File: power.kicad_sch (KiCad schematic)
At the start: 27 parts, among them J14 DeployLipo, J15 UCLipo, Q10 AO3401A, Q7 SI4143DY-T1-GE3, Q8 SI4143DY-T1-GE3, Q9 AO3401A, U10 LTC4411ES5TRMPBF, U11 LTC4411ES5TRMPBF, U12 LT1963AxST-3.3, U13 LTC4412xS6, U14 LTC4412xS6, U15 LTC4412xS6, U16 LTC4412xS6

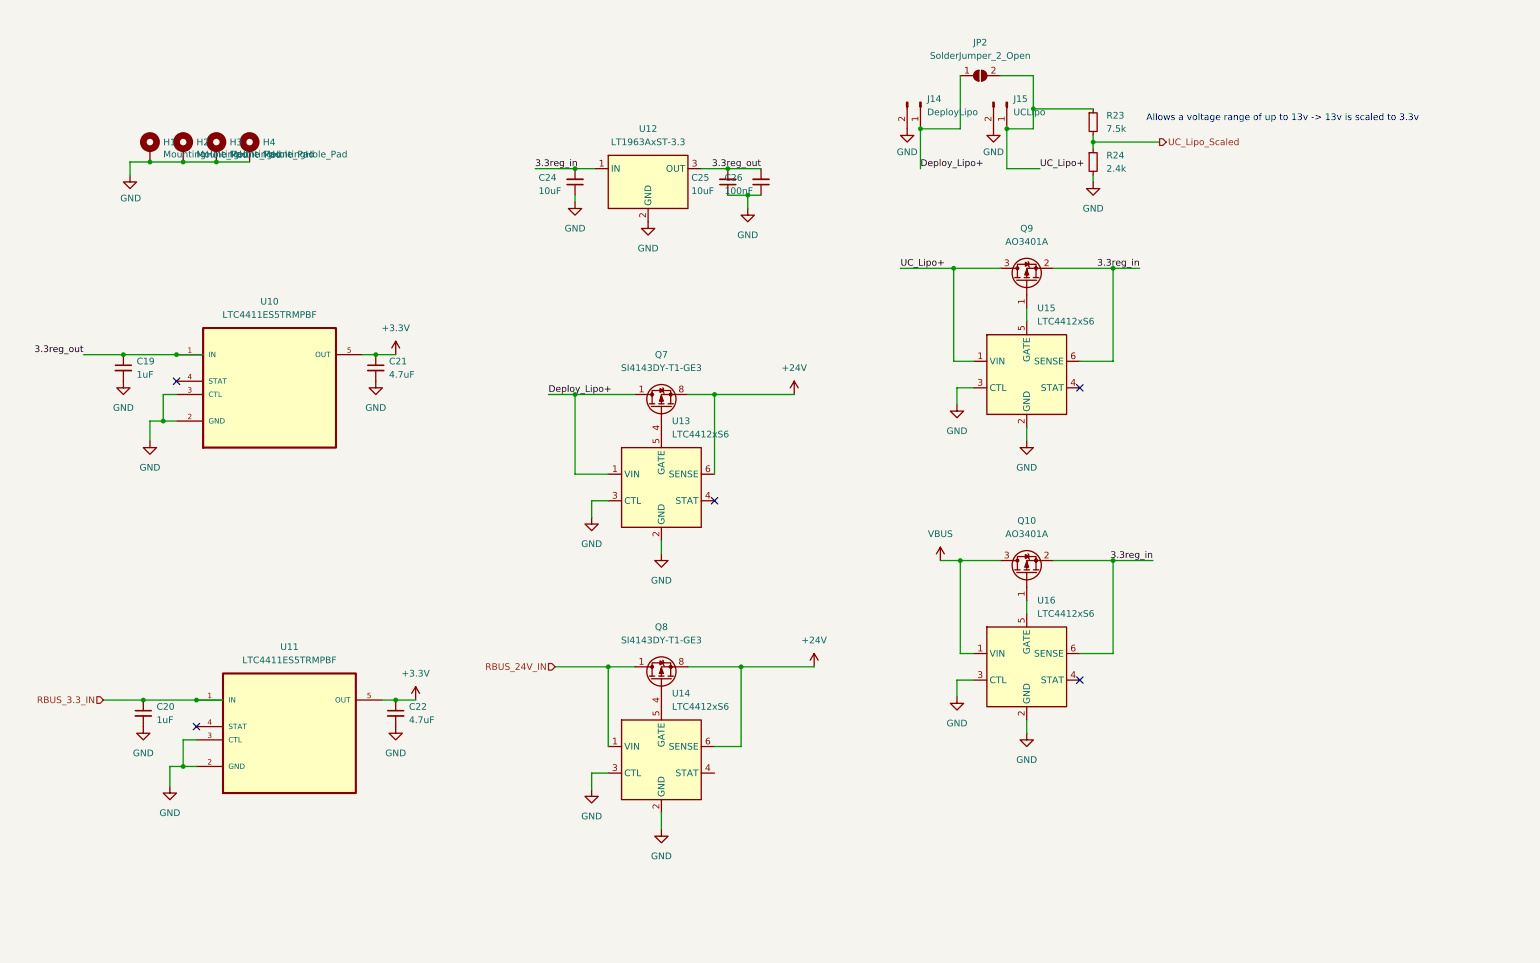
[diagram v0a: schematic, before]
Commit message: working on v2
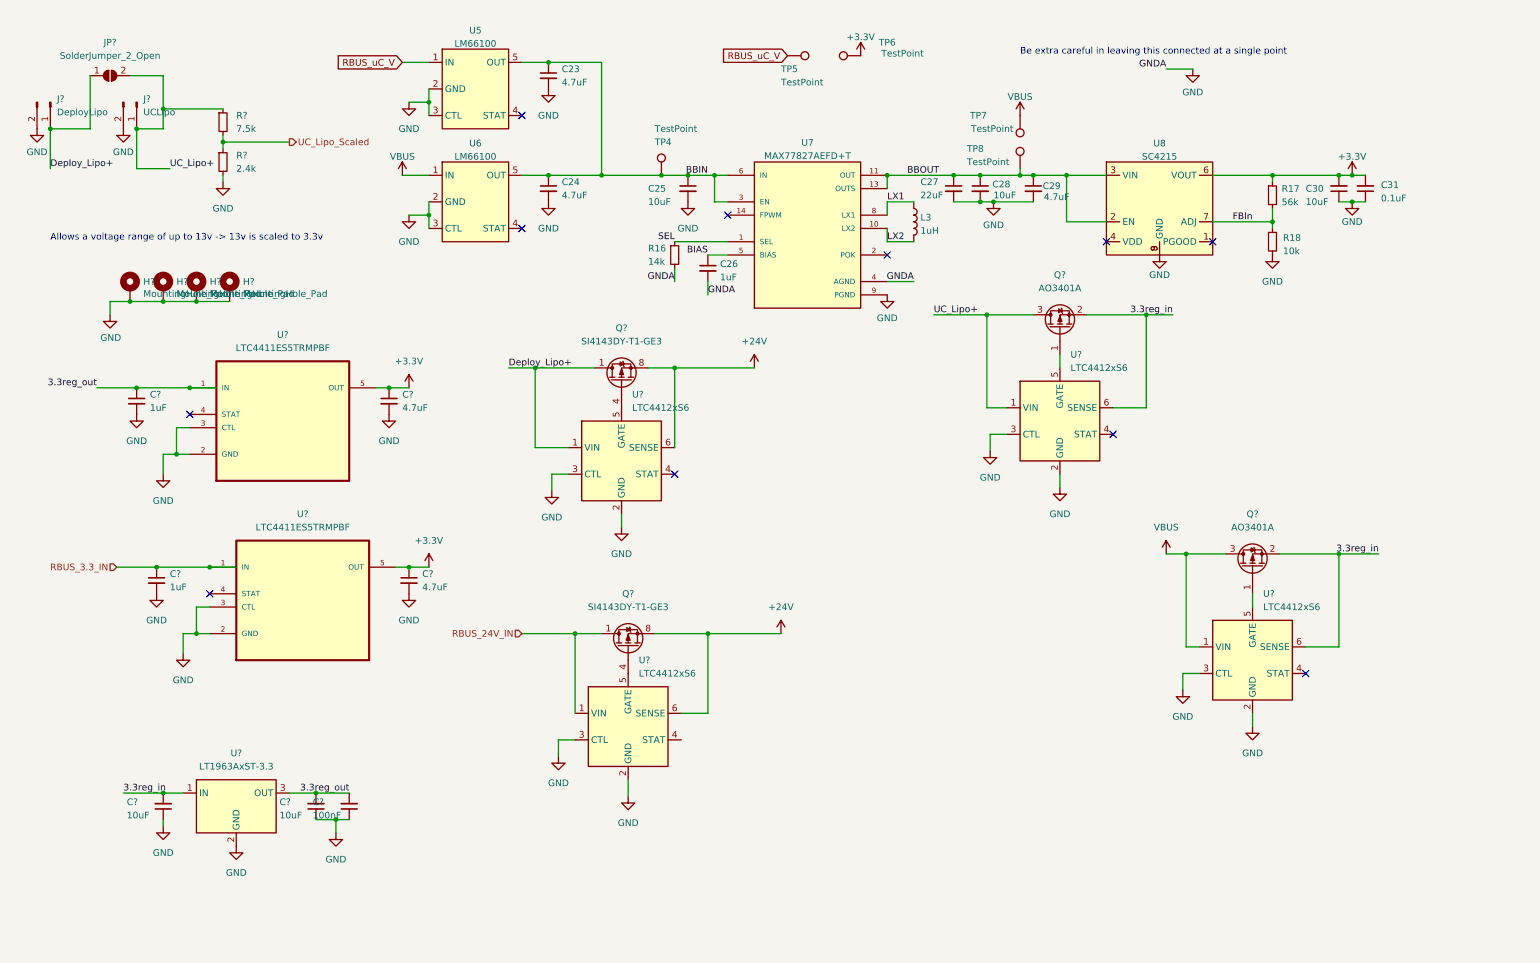
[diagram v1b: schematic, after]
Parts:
- removed C19, C20: 1uF, Capacitor_SMD:C_0603_1608Metric, symbol Device:C_Small
- removed C21, C22: 4.7uF, Capacitor_SMD:C_0603_1608Metric, symbol Device:C_Small
- removed H1, H2, H3, H4: MountingHole_Pad, MountingHole:MountingHole_3.2mm_M3_DIN965_Pad, symbol Mechanical:MountingHole_Pad
- removed J14: DeployLipo, TerminalBlock_Phoenix:TerminalBlock_Phoenix_MKDS-3-2-5.08_1x02_P5.08mm_Horizontal, symbol Connector:Conn_01x02_Male
- removed J15: UCLipo, Connector_JST:JST_PH_B2B-PH-K_1x02_P2.00mm_Vertical, symbol Connector:Conn_01x02_Male
- removed JP2: SolderJumper_2_Open, Jumper:SolderJumper-2_P1.3mm_Open_RoundedPad1.0x1.5mm, symbol Jumper:SolderJumper_2_Open
- removed Q10, Q9: AO3401A, Package_TO_SOT_SMD:SOT-23, symbol Transistor_FET:AO3401A
- removed Q7, Q8: SI4143DY-T1-GE3, Package_SO:SOIC-8_3.9x4.9mm_P1.27mm, symbol Device:Q_PMOS_GDS
- removed R23: 7.5k, Resistor_SMD:R_0603_1608Metric, symbol Device:R_Small
- removed R24: 2.4k, Resistor_SMD:R_0603_1608Metric, symbol Device:R_Small
- removed U10, U11: LTC4411ES5TRMPBF, Package_TO_SOT_SMD:SOT-23-5_HandSoldering, symbol LTC4411ES5TRMPBF:LTC4411ES5TRMPBF
- removed U12: LT1963AxST-3.3, Package_TO_SOT_SMD:SOT-223-3_TabPin2, symbol Regulator_Linear:LT1963AxST-3.3
- removed U13, U14, U15, U16: LTC4412xS6, Package_TO_SOT_SMD:TSOT-23-6, symbol Power_Management:LTC4412xS6
- added C23, C29: 4.7uF, Capacitor_SMD:C_0402_1005Metric, symbol Device:C_Small
- added C27: 22uF, Capacitor_SMD:C_0603_1608Metric, symbol Device:C_Small
- added C28, C30: 10uF, Capacitor_SMD:C_0402_1005Metric, symbol Device:C_Small
- added C31: 0.1uF, Capacitor_SMD:C_0402_1005Metric, symbol Device:C_Small
- added C? (x2): 1uF, Capacitor_SMD:C_0603_1608Metric, symbol Device:C_Small
- added C? (x2): 10uF, Capacitor_SMD:C_0603_1608Metric, symbol Device:C_Small
- added C? (x2): 4.7uF, Capacitor_SMD:C_0603_1608Metric, symbol Device:C_Small
- added C?: 100nF, Capacitor_SMD:C_0603_1608Metric, symbol Device:C_Small
- added H? (x4): MountingHole_Pad, MountingHole:MountingHole_3.2mm_M3_DIN965_Pad, symbol Mechanical:MountingHole_Pad
- added J?: UCLipo, Connector_JST:JST_PH_B2B-PH-K_1x02_P2.00mm_Vertical, symbol Connector:Conn_01x02_Male
- added J?: DeployLipo, TerminalBlock_Phoenix:TerminalBlock_Phoenix_MKDS-3-2-5.08_1x02_P5.08mm_Horizontal, symbol Connector:Conn_01x02_Male
- added JP?: SolderJumper_2_Open, Jumper:SolderJumper-2_P1.3mm_Open_RoundedPad1.0x1.5mm, symbol Jumper:SolderJumper_2_Open
- added L3: 1uH, Inductor_SMD:L_0805_2012Metric, symbol Device:L
- added Q? (x2): AO3401A, Package_TO_SOT_SMD:SOT-23, symbol Transistor_FET:AO3401A
- added Q? (x2): SI4143DY-T1-GE3, Package_SO:SOIC-8_3.9x4.9mm_P1.27mm, symbol Device:Q_PMOS_GDS
- added R16: 14k, Resistor_SMD:R_0402_1005Metric, symbol Device:R_Small
- added R17: 56k, Resistor_SMD:R_0402_1005Metric, symbol Device:R_Small
- added R18: 10k, Resistor_SMD:R_0402_1005Metric, symbol Device:R_Small
- added R?: 7.5k, Resistor_SMD:R_0603_1608Metric, symbol Device:R_Small
- added R?: 2.4k, Resistor_SMD:R_0603_1608Metric, symbol Device:R_Small
- added TP4, TP5, TP6, TP7, TP8: TestPoint, TestPoint:TestPoint_Pad_D1.5mm, symbol Connector:TestPoint
- added U5, U6: LM66100, Package_TO_SOT_SMD:SOT-23-5, symbol iclr:LTC4411
- added U7: MAX77827AEFD+T, iclr:CONV_MAX77827AEFD+T, symbol iclr:MAX77827AEFD+T
- added U8: SC4215, iclr:SOIC127P599X175-9N, symbol iclr:RT9025-25GSP
- added U? (x2): LTC4411ES5TRMPBF, Package_TO_SOT_SMD:SOT-23-5_HandSoldering, symbol LTC4411ES5TRMPBF:LTC4411ES5TRMPBF
- added U? (x4): LTC4412xS6, Package_TO_SOT_SMD:TSOT-23-6, symbol Power_Management:LTC4412xS6
- added U?: LT1963AxST-3.3, Package_TO_SOT_SMD:SOT-223-3_TabPin2, symbol Regulator_Linear:LT1963AxST-3.3
- C24: value 10uF -> 4.7uF; footprint Capacitor_SMD:C_0603_1608Metric -> Capacitor_SMD:C_0402_1005Metric
- C26: value 100nF -> 1uF; footprint Capacitor_SMD:C_0603_1608Metric -> Capacitor_SMD:C_0402_1005Metric
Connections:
- net +24V: now also Q?.5 (D), Q?.5 (D), Q?.6 (D), Q?.6 (D), Q?.7 (D), Q?.7 (D), Q?.8 (D), Q?.8 (D), U?.6 (SENSE), U?.6 (SENSE)
- net +3V3: now also C30.2, C31.2, C?.1, C?.1, R17.1, TP6.1, U8.6 (VOUT), U?.5 (OUT), U?.5 (OUT)
- net 3.3reg_in: now also C?.2, Q?.2 (S), Q?.2 (S), U?.1 (IN), U?.6 (SENSE), U?.6 (SENSE); no longer C24.2
- net 3.3reg_out: now also C?.1, C?.2, C?.2, U?.1 (IN), U?.3 (OUT); no longer C25.2, C26.2
- net Deploy_Lipo+: now also J?.1 (Pin_1), JP?.1 (A), Q?.1 (S), Q?.2 (S), Q?.3 (S), U?.1 (VIN)
- net GND: now also C24.2, C25.2, C26.2, C23.2, C27.2, C28.2, C29.2, C30.1, C31.1, C?.1, C?.1, C?.1, C?.2, C?.2, C?.2, C?.2, H?.1, H?.1, H?.1, H?.1, J?.2 (Pin_2), J?.2 (Pin_2), R16.2, R18.2, R?.2, U5.2 (GND), U5.3 (CTL), U6.2 (GND), U6.3 (CTL), U7.4 (AGND), U7.9 (PGND), U8.8 (GND), U8.9 (GND), U?.2 (GND), U?.2 (GND), U?.2 (GND), U?.2 (GND), U?.2 (GND), U?.2 (GND), U?.2 (GND), U?.3 (CTL), U?.3 (CTL), U?.3 (CTL), U?.3 (CTL), U?.3 (CTL), U?.3 (CTL); no longer C24.1, C25.1, C26.1
- net RBUS_24V_IN: now also Q?.1 (S), Q?.2 (S), Q?.3 (S), U?.1 (VIN)
- net RBUS_3.3_IN: now also C?.1, U?.1 (IN)
- net UC_Lipo+: now also J?.1 (Pin_1), JP?.2 (B), Q?.3 (D), R?.1, U?.1 (VIN)
- net UC_Lipo_Scaled: now also R?.1, R?.2
- net VBUS: now also Q?.3 (D), TP7.1, U6.1 (IN), U?.1 (VIN)
- new net: Q?.1 (G), U?.5 (GATE) (x2)
- new net: Q?.4 (G), U?.5 (GATE) (x2)
- new net BBIN: C23.1, C24.1, C25.1, TP4.1, U5.5 (OUT), U6.5 (OUT), U7.3 (EN), U7.6 (IN)
- new net BBOUT: C27.1, C28.1, C29.1, TP8.1, U7.11 (OUT), U7.13 (OUTS), U8.2 (EN), U8.3 (VIN)
- new net BIAS: C26.1, U7.5 (BIAS)
- new net FBIn: R17.2, R18.1, U8.7 (ADJ)
- new net LX1: L3.1, U7.8 (LX1)
- new net LX2: L3.2, U7.10 (LX2)
- new net RBUS_uC_V: TP5.1, U5.1 (IN)
- new net SEL: R16.1, U7.1 (SEL)
- no-connect marks 5 -> 11
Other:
- note added: "Be extra careful in leaving this connected at a single point"

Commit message: v2 time
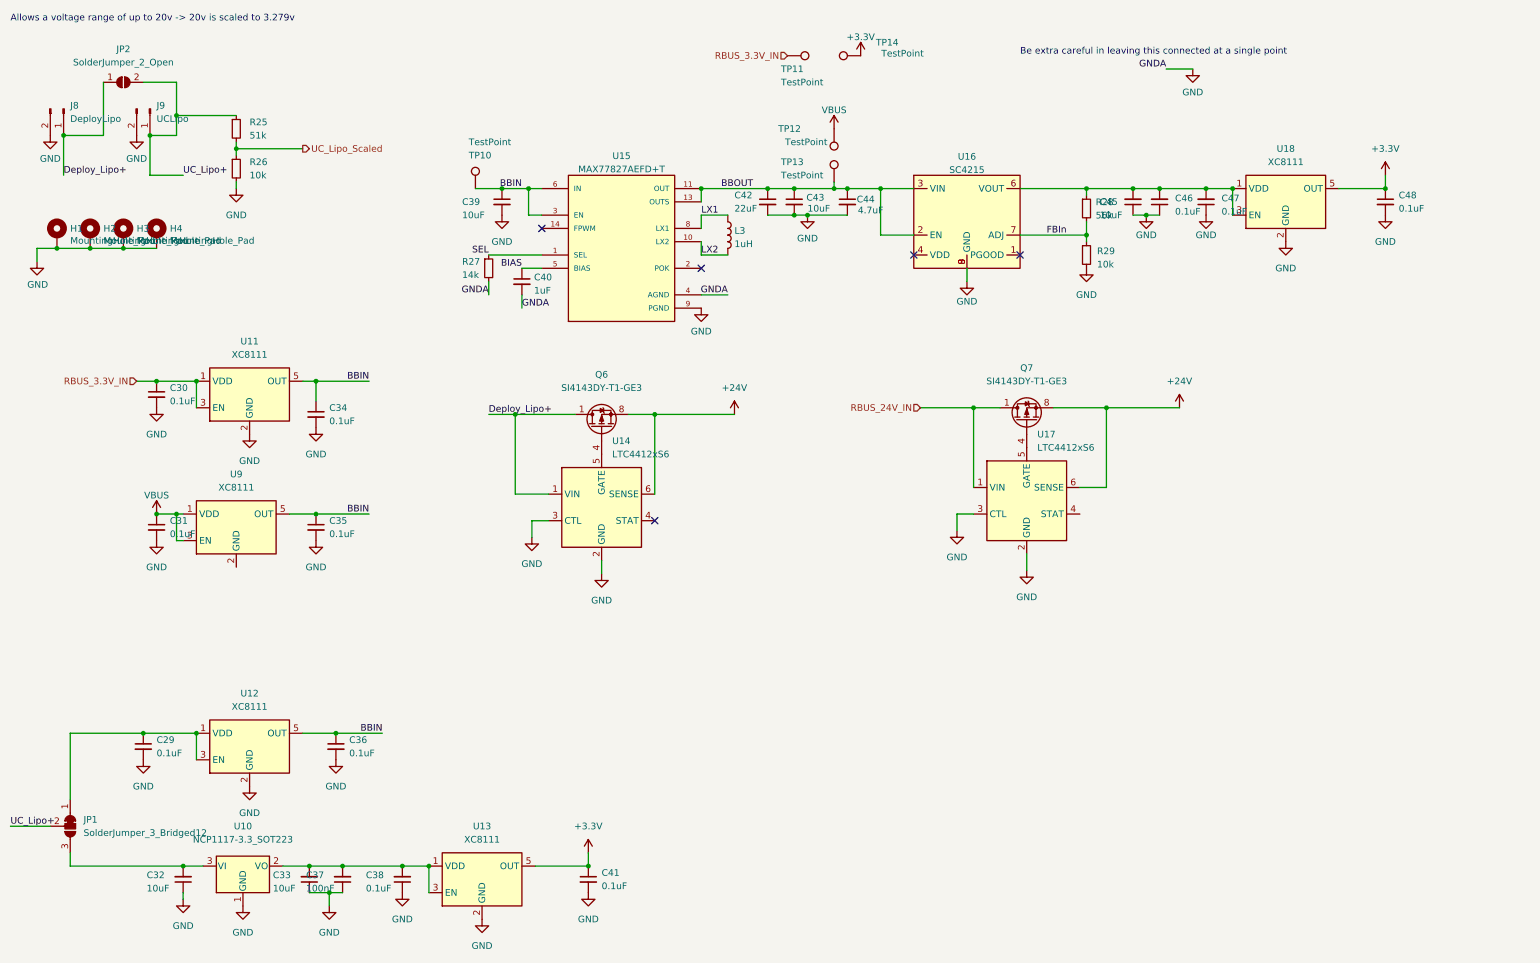
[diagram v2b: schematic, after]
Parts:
- removed C24: 4.7uF, Capacitor_SMD:C_0402_1005Metric, symbol Device:C_Small
- removed C? (x2): 1uF, Capacitor_SMD:C_0603_1608Metric, symbol Device:C_Small
- removed C? (x2): 4.7uF, Capacitor_SMD:C_0603_1608Metric, symbol Device:C_Small
- removed Q? (x2): AO3401A, Package_TO_SOT_SMD:SOT-23, symbol Transistor_FET:AO3401A
- removed U5, U6: LM66100, Package_TO_SOT_SMD:SOT-23-5, symbol iclr:LTC4411
- removed U? (x2): LTC4411ES5TRMPBF, Package_TO_SOT_SMD:SOT-23-5_HandSoldering, symbol LTC4411ES5TRMPBF:LTC4411ES5TRMPBF
- removed U? (x2): LTC4412xS6, Package_TO_SOT_SMD:TSOT-23-6, symbol Power_Management:LTC4412xS6
- removed U?: LT1963AxST-3.3, Package_TO_SOT_SMD:SOT-223-3_TabPin2, symbol Regulator_Linear:LT1963AxST-3.3
- added C29, C30, C31, C35, C36, C38, C41, C47, C48: 0.1uF, Capacitor_SMD:C_0402_1005Metric, symbol Device:C_Small
- added JP1: SolderJumper_3_Bridged12, Jumper:SolderJumper-3_P1.3mm_Bridged12_RoundedPad1.0x1.5mm, symbol Jumper:SolderJumper_3_Bridged12
- added U10: NCP1117-3.3_SOT223, Package_TO_SOT_SMD:SOT-223-3_TabPin2, symbol Regulator_Linear:NCP1117-3.3_SOT223
- added U11, U12, U13, U18, U9: XC8111, Package_TO_SOT_SMD:SOT-23-5, symbol Analog_Switch:MAX40200AUK
- C32, C33, C37: renamed from C?; footprint Capacitor_SMD:C_0603_1608Metric -> Capacitor_SMD:C_0402_1005Metric
- C34: renamed from C23; value 4.7uF -> 0.1uF
- R25: renamed from R?; value 7.5k -> 51k; footprint Resistor_SMD:R_0603_1608Metric -> Resistor_SMD:R_0402_1005Metric
- R26: renamed from R?; value 2.4k -> 10k; footprint Resistor_SMD:R_0603_1608Metric -> Resistor_SMD:R_0402_1005Metric
- gave numbers to parts that had none: 11
- renumbered C25 to C39, C26 to C40, C27 to C42, C28 to C43, C29 to C44, C30 to C45, C31 to C46, R16 to R27, R17 to R28, R18 to R29, TP4 to TP10, TP5 to TP11, TP7 to TP12, TP8 to TP13, TP6 to TP14, U7 to U15, U8 to U16
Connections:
- net +3V3: now also C41.1, C48.1, U13.5 (OUT), U18.5 (OUT); no longer C45.2, C46.2, R28.1, U16.6 (VOUT)
- net BBIN: now also C35.1, C36.1, U11.5 (OUT), U12.5 (OUT), U9.5 (OUT)
- net GND: now also C29.2, C30.2, C31.2, C35.2, C36.2, C38.1, C41.2, C47.1, C48.2, U10.1 (GND), U11.2 (GND), U12.2 (GND), U13.2 (GND), U18.2 (GND)
- net UC_Lipo+: now also JP1.2 (C)
- net VBUS: now also C31.1, U9.1 (VDD), U9.3 (EN)
- net 3.3reg_in: no longer names the net of C32.2
- net 3.3reg_in: now also JP1.3 (B), U10.3 (VI)
- net 3.3reg_out: no longer names the net of C33.2, C37.2
- net 3.3reg_out: now also C38.2, U10.2 (VO), U13.1 (VDD), U13.3 (EN)
- net RBUS_uC_V renamed RBUS_3.3V_IN
- net RBUS_3.3V_IN: now also C30.1, U11.1 (VDD), U11.3 (EN)
- new net: C45.2, C46.2, C47.2, R28.1, U16.6 (VOUT), U18.1 (VDD), U18.3 (EN)
- new net: C29.1, JP1.1 (A), U12.1 (VDD), U12.3 (EN)
- no-connect marks 11 -> 5
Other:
- note added: "Allows a voltage range of up to 20v -> 20v is scaled to 3.279v"
- note removed: "Allows a voltage range of up to 13v -> 13v is scaled to 3.3v"
- moved on the sheet: C32, C33, C34, C37, C39, C40, C42, C43, C44, C45, C46, H1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
